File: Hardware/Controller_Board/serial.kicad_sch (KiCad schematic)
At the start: 28 parts, among them U501 FT232H, U502 93LC56B, Y2 12MHz

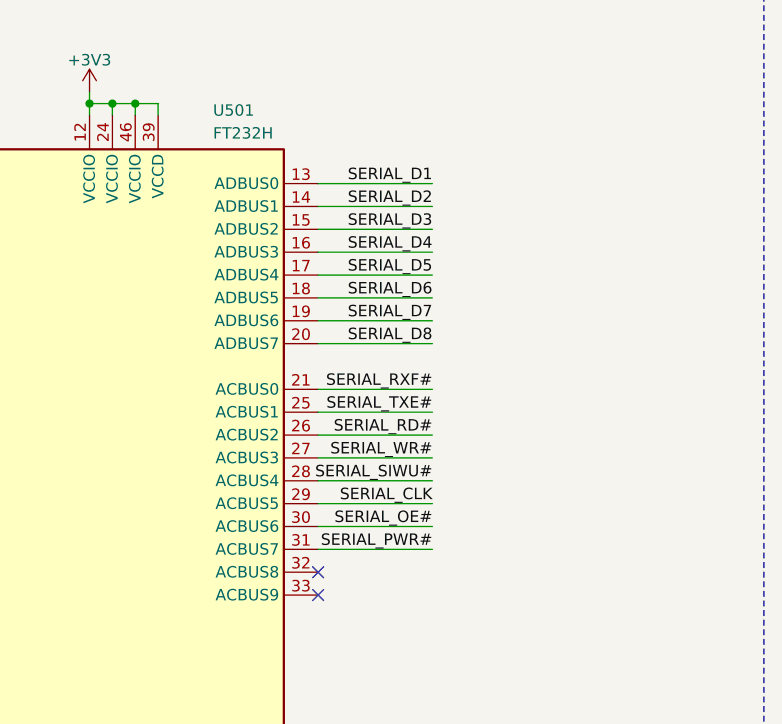
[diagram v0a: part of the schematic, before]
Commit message: Advanced PCB design: Routed FTDIs + SPI Flash
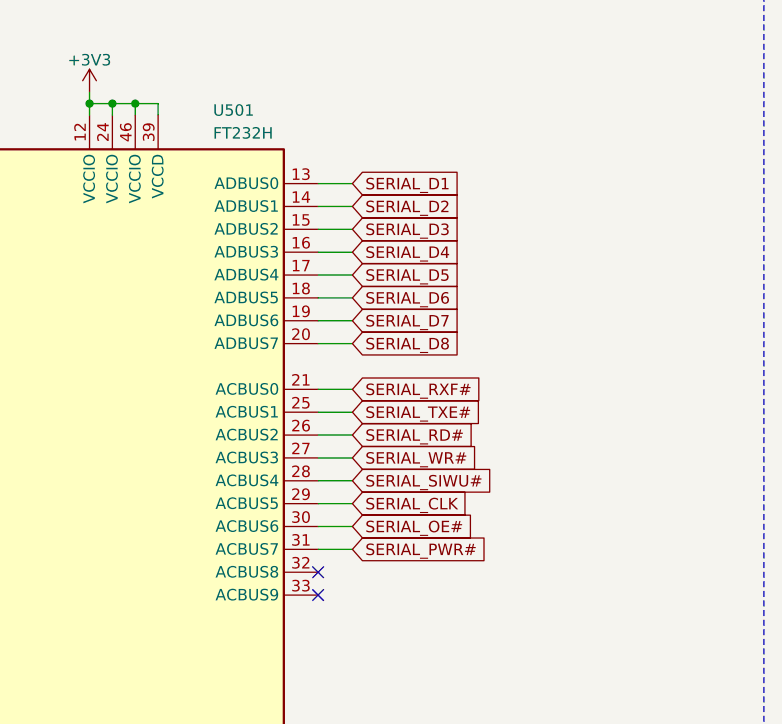
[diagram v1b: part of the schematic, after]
